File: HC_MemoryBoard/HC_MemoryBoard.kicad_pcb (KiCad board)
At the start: 2 copper layers, 100 x 100 mm, 607 parts, among them IC1 HM62256BLP, IC2 74HC30, IC3 74HC138, IC4 74HC32, IC5 74HC541, J1 Expantion_Connector, J2 Conn_01x02_Pin, J3 Conn_01x08_Pin, J4 Expantion_Connector, J5 Conn_01x08_Pin, J6 Conn_01x02_Pin, J7 Conn_01x02_Pin, SW1 SW_DIP_x08

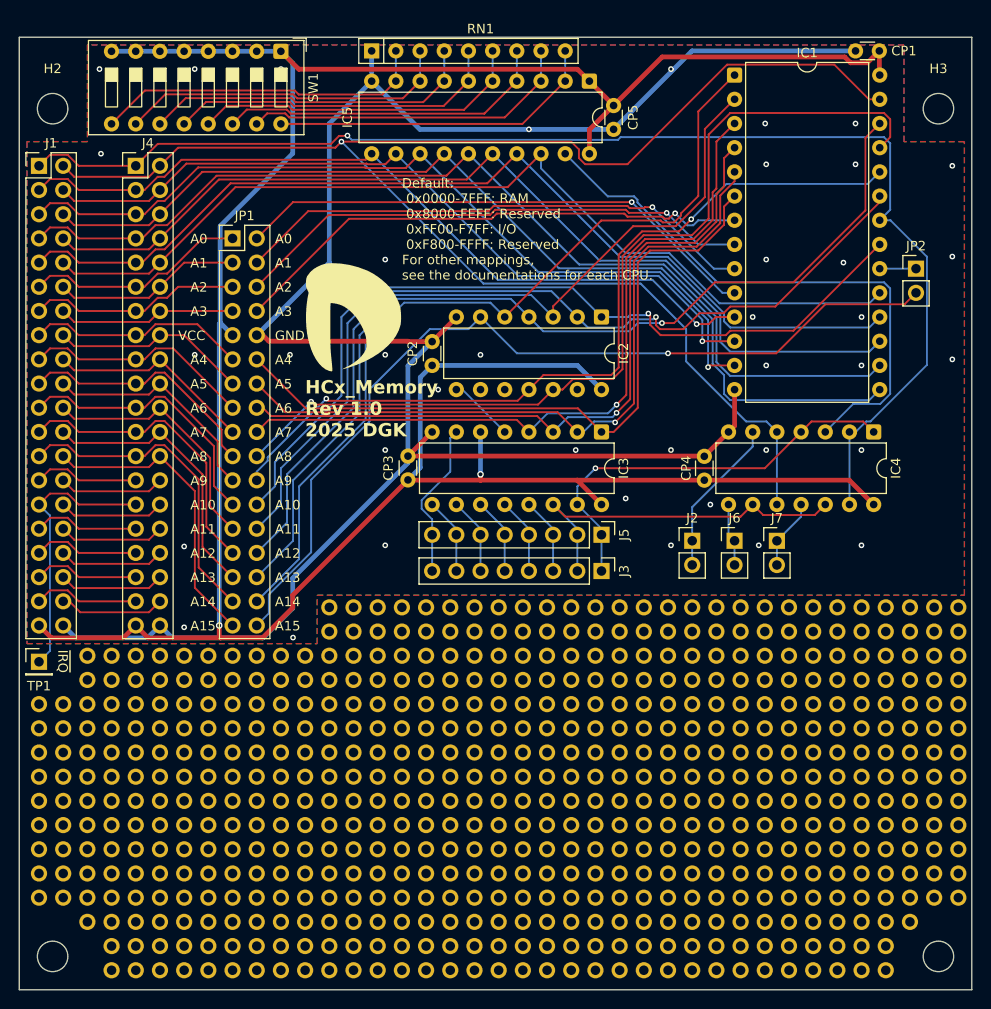
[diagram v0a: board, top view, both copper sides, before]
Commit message: Memboardv2.0
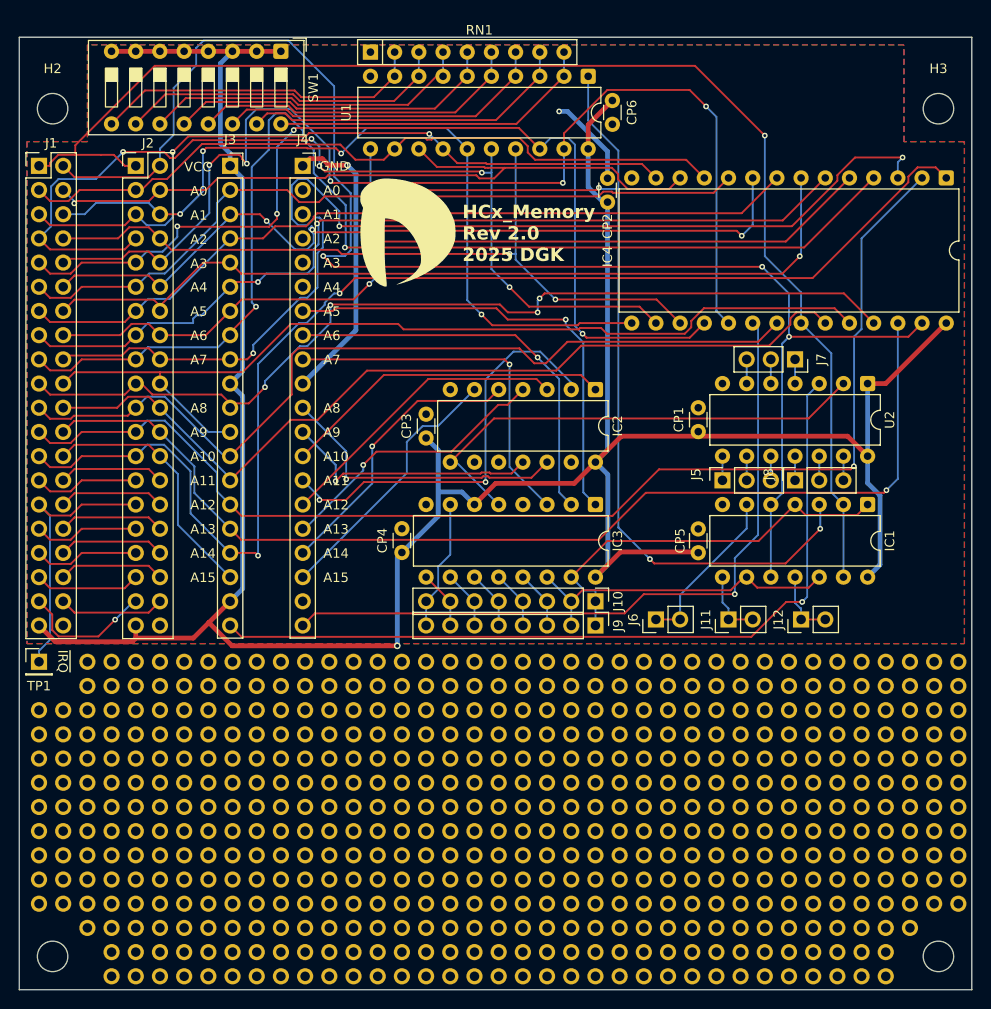
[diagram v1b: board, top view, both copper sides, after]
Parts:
- removed IC5: 74HC541, Package_DIP:DIP-20_W7.62mm
- removed JP1: Conn_02x17_Counter_Clockwise, Connector_PinHeader_2.54mm:PinHeader_2x17_P2.54mm_Vertical
- removed JP2: Jumper_2_Bridged, Connector_PinHeader_2.54mm:PinHeader_1x02_P2.54mm_Vertical
- removed REF** (x4): ThroughHole_d1.0_D1.7, ThroughHole:ThroughHole_d1.0_D1.7
- removed the REF**14 at (85.1, 114.9)
- removed the REF**14 at (82.5, 112.4)
- removed the REF**14 at (82.5, 109.9)
- removed the REF**15 at (87.6, 114.9)
- removed the REF**15 at (85.1, 112.4)
- removed the REF**15 at (85.1, 109.9)
- removed the REF**16 at (87.6, 112.4)
- removed the REF**16 at (87.6, 109.9)
- removed the REF**16 at (90.2, 114.9)
- removed the REF**17 at (92.7, 114.9)
- removed the REF**17 at (90.2, 112.4)
- removed the REF**17 at (90.2, 109.9)
- removed the REF**18 at (92.7, 112.4)
- removed the REF**18 at (95.2, 114.9)
- removed the REF**18 at (92.7, 109.9)
- removed the REF**19 at (95.2, 109.9)
- removed the REF**19 at (95.2, 112.4)
- removed the REF**19 at (97.8, 114.9)
- removed the REF**20 at (97.8, 112.4)
- removed the REF**20 at (97.8, 109.9)
- removed the REF**20 at (100.3, 114.9)
- removed the REF**21 at (100.3, 109.9)
- removed the REF**21 at (102.9, 114.9)
- removed the REF**21 at (100.3, 112.4)
- removed the REF**22 at (102.9, 112.4)
- removed the REF**22 at (102.9, 109.9)
- removed the REF**22 at (105.4, 114.9)
- removed the REF**23 at (108.0, 114.9)
- removed the REF**23 at (105.4, 112.4)
- removed the REF**23 at (105.4, 109.9)
- removed the REF**24 at (108.0, 109.9)
- removed the REF**24 at (110.5, 114.9)
- removed the REF**24 at (108.0, 112.4)
- removed the REF**25 at (110.5, 109.9)
- removed the REF**25 at (110.5, 112.4)
- removed the REF**25 at (113.0, 114.9)
- removed the REF**26 at (113.0, 112.4)
- removed the REF**26 at (113.0, 109.9)
- removed the REF**26 at (115.6, 114.9)
- removed the REF**27 at (115.6, 109.9)
- removed the REF**27 at (115.6, 112.4)
- removed the REF**27 at (118.1, 114.9)
- removed the REF**28 at (118.1, 112.4)
- removed the REF**28 at (118.1, 109.9)
- removed the REF**28 at (120.7, 114.9)
- removed the REF**29 at (123.2, 114.9)
- removed the REF**29 at (120.7, 109.9)
- removed the REF**29 at (120.7, 112.4)
- removed the REF**30 at (125.7, 114.9)
- removed the REF**30 at (123.2, 109.9)
- removed the REF**30 at (123.2, 112.4)
- removed the REF**31 at (128.3, 114.9)
- removed the REF**31 at (125.7, 109.9)
- removed the REF**31 at (125.7, 112.4)
- removed the REF**32 at (130.8, 114.9)
- removed the REF**32 at (128.3, 109.9)
- removed the REF**32 at (128.3, 112.4)
- removed the REF**33 at (130.8, 112.4)
- removed the REF**33 at (130.8, 109.9)
- removed the REF**33 at (133.3, 114.9)
- removed the REF**34 at (133.3, 109.9)
- removed the REF**34 at (135.9, 114.9)
- removed the REF**34 at (133.3, 112.4)
- removed the REF**35 at (138.4, 114.9)
- removed the REF**35 at (135.9, 109.9)
- removed the REF**35 at (135.9, 112.4)
- removed the REF**36 at (138.4, 109.9)
- removed the REF**36 at (138.4, 112.4)
- removed the REF**36 at (141.0, 114.9)
- removed the REF**37 at (141.0, 109.9)
- removed the REF**37 at (141.0, 112.4)
- removed the REF**37 at (143.5, 114.9)
- removed the REF**38 at (143.5, 112.4)
- removed the REF**38 at (146.1, 114.9)
- removed the REF**38 at (143.5, 109.9)
- removed the REF**39 at (146.1, 112.4)
- removed the REF**39 at (148.6, 114.9)
- removed the REF**39 at (146.1, 109.9)
- added CP1: 0.1u, Capacitor_THT:C_Disc_D3.0mm_W1.6mm_P2.50mm, F.Cu at (121.3, 91.4)
- added J3: Changer, Connector_PinSocket_2.54mm:PinSocket_1x20_P2.54mm_Vertical, F.Cu at (72.1, 63.5)
- added J4: Changer, Connector_PinSocket_2.54mm:PinSocket_1x20_P2.54mm_Vertical, F.Cu at (79.8, 63.5)
- added J5: Conn_01x03_Pin, Connector_PinSocket_2.54mm:PinSocket_1x03_P2.54mm_Vertical, F.Cu at (123.8, 96.5)
- added J7: Conn_01x03_Pin, Connector_PinSocket_2.54mm:PinSocket_1x03_P2.54mm_Vertical, F.Cu at (131.4, 83.8)
- added J8: Conn_01x03_Pin, Connector_PinSocket_2.54mm:PinSocket_1x03_P2.54mm_Vertical, F.Cu at (131.4, 96.5)
- added REF**14: ThroughHole_d1.0_D1.7, ThroughHole:ThroughHole_d1.0_D1.7, F.Cu at (85.1, 115.6)
- added REF**15: ThroughHole_d1.0_D1.7, ThroughHole:ThroughHole_d1.0_D1.7, F.Cu at (87.6, 115.6)
- added REF**16: ThroughHole_d1.0_D1.7, ThroughHole:ThroughHole_d1.0_D1.7, F.Cu at (90.2, 115.6)
- added REF**17: ThroughHole_d1.0_D1.7, ThroughHole:ThroughHole_d1.0_D1.7, F.Cu at (92.7, 115.6)
- added REF**18: ThroughHole_d1.0_D1.7, ThroughHole:ThroughHole_d1.0_D1.7, F.Cu at (95.2, 115.6)
- added REF**19: ThroughHole_d1.0_D1.7, ThroughHole:ThroughHole_d1.0_D1.7, F.Cu at (97.8, 115.6)
- added REF**20: ThroughHole_d1.0_D1.7, ThroughHole:ThroughHole_d1.0_D1.7, F.Cu at (100.3, 115.6)
- added REF**21: ThroughHole_d1.0_D1.7, ThroughHole:ThroughHole_d1.0_D1.7, F.Cu at (102.9, 115.6)
- added REF**22: ThroughHole_d1.0_D1.7, ThroughHole:ThroughHole_d1.0_D1.7, F.Cu at (105.4, 115.6)
- added REF**23: ThroughHole_d1.0_D1.7, ThroughHole:ThroughHole_d1.0_D1.7, F.Cu at (108.0, 115.6)
- added REF**24: ThroughHole_d1.0_D1.7, ThroughHole:ThroughHole_d1.0_D1.7, F.Cu at (110.5, 115.6)
- added REF**25: ThroughHole_d1.0_D1.7, ThroughHole:ThroughHole_d1.0_D1.7, F.Cu at (113.0, 115.6)
- added REF**26: ThroughHole_d1.0_D1.7, ThroughHole:ThroughHole_d1.0_D1.7, F.Cu at (115.6, 115.6)
- added REF**27: ThroughHole_d1.0_D1.7, ThroughHole:ThroughHole_d1.0_D1.7, F.Cu at (118.1, 115.6)
- added REF**28: ThroughHole_d1.0_D1.7, ThroughHole:ThroughHole_d1.0_D1.7, F.Cu at (120.7, 115.6)
- added REF**29: ThroughHole_d1.0_D1.7, ThroughHole:ThroughHole_d1.0_D1.7, F.Cu at (123.2, 115.6)
- added REF**30: ThroughHole_d1.0_D1.7, ThroughHole:ThroughHole_d1.0_D1.7, F.Cu at (125.7, 115.6)
- added REF**31: ThroughHole_d1.0_D1.7, ThroughHole:ThroughHole_d1.0_D1.7, F.Cu at (128.3, 115.6)
- added REF**32: ThroughHole_d1.0_D1.7, ThroughHole:ThroughHole_d1.0_D1.7, F.Cu at (130.8, 115.6)
- added REF**33: ThroughHole_d1.0_D1.7, ThroughHole:ThroughHole_d1.0_D1.7, F.Cu at (133.3, 115.6)
- added REF**34: ThroughHole_d1.0_D1.7, ThroughHole:ThroughHole_d1.0_D1.7, F.Cu at (135.9, 115.6)
- added REF**35: ThroughHole_d1.0_D1.7, ThroughHole:ThroughHole_d1.0_D1.7, F.Cu at (138.4, 115.6)
- added REF**36: ThroughHole_d1.0_D1.7, ThroughHole:ThroughHole_d1.0_D1.7, F.Cu at (141.0, 115.6)
- added REF**37: ThroughHole_d1.0_D1.7, ThroughHole:ThroughHole_d1.0_D1.7, F.Cu at (143.5, 115.6)
- added REF**38: ThroughHole_d1.0_D1.7, ThroughHole:ThroughHole_d1.0_D1.7, F.Cu at (146.1, 115.6)
- added REF**39: ThroughHole_d1.0_D1.7, ThroughHole:ThroughHole_d1.0_D1.7, F.Cu at (148.6, 115.6)
- added REF**432: ThroughHole_d1.0_D1.7, ThroughHole:ThroughHole_d1.0_D1.7, F.Cu at (57.1, 143.5)
- added REF**466: ThroughHole_d1.0_D1.7, ThroughHole:ThroughHole_d1.0_D1.7, F.Cu at (143.5, 143.5)
- added U1: 74HC573, Package_DIP:DIP-20_W7.62mm, F.Cu at (109.7, 54.1)
- added U2: 74HC00, Package_DIP:DIP-14_W7.62mm, F.Cu at (139.1, 86.4)
- moved CP2 32.7 mm to (111.8, 67.3), turned to 90 degrees
- moved IC4 24.7 mm to (147.3, 64.8), turned to -90 degrees
- moved G*** 10.6 mm to (90.8, 70.5)
- moved J6 9.10 mm to (116.8, 111.1), turned to 90 degrees
- moved J12 8.64 mm to (132.1, 111.1), turned to 90 degrees
- moved J11 8.28 mm to (124.5, 111.1), turned to 90 degrees
- moved CP3 7.65 mm to (92.7, 92.1)
- moved CP4 7.65 mm to (90.2, 104.1)
- moved CP5 7.65 mm to (121.3, 104.1)
- moved IC3 7.65 mm to (110.5, 99.1)
- moved IC1 7.65 mm to (139.1, 99.1)
- moved IC2 7.65 mm to (110.5, 87.0)
- moved J10 7.01 mm to (110.5, 109.2)
- moved J9 5.76 mm to (110.5, 111.8)
- moved REF**352 0.64 mm to (52.1, 138.4)
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- renumbered CP1 to CP2, CP2 to CP3, CP3 to CP4, CP4 to CP5, CP5 to CP6, IC4 to IC1, IC1 to IC4, J5 to J10, J6 to J11, J7 to J12, J4 to J2, J2 to J6, J3 to J9
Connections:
- net Net-(IC3-~{E1}) renamed /7430
- IC3 pad 1: /A4 -> /A5
- IC3 pad 2: /A5 -> /A6
- IC3 pad 3: /A6 -> /A7
- IC3 pad 4: /A7 -> GND
- IC4 pad 1: /A14 -> /AD14
- IC4 pad 10: /A0 -> /AD0
- IC4 pad 2: /A12 -> /AD12
- IC4 pad 20: Net-(IC1-~{CS}) -> /~{RAM_CE}
- IC4 pad 21: /A10 -> /AD10
- IC4 pad 23: /A11 -> /AD11
- IC4 pad 24: /A9 -> /AD9
- IC4 pad 25: /A8 -> /AD8
- IC4 pad 26: /A13 -> /AD13
- IC4 pad 3: /A7 -> /AD7
- IC4 pad 4: /A6 -> /AD6
- IC4 pad 5: /A5 -> /AD5
- IC4 pad 6: /A4 -> /AD4
- IC4 pad 7: /A3 -> /AD3
- IC4 pad 8: /A2 -> /AD2
- IC4 pad 9: /A1 -> /AD1
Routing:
- net GND: track 217.6 -> 40.5 mm, vias 39 -> 2
- net /AD14: track 34.0 -> 133.7 mm, vias 0 -> 2
- net /AD6: track 24.3 -> 124.0 mm, vias 0 -> 2
- net /AD7: track 21.9 -> 119.1 mm, vias 0 -> 3
- net /AD12: track 31.4 -> 127.7 mm, vias 0 -> 1
- net Net-(J3-Pin_20): track 0.00 -> 85.7 mm, vias 0 -> 1
- net /AD13: track 29.5 -> 113.9 mm, vias 0 -> 1
- net /~{RAM_CE}: track 0.00 -> 76.4 mm, vias 0 -> 1
- net /AD9: track 24.4 -> 98.5 mm
- net /A4: track 73.6 -> 0.00 mm
- net /AD5: track 20.8 -> 93.4 mm, vias 0 -> 2
- net /AD8: track 26.3 -> 98.9 mm, vias 0 -> 4
- net /A13: track 101.0 -> 29.5 mm
- net /AD3: track 18.7 -> 90.0 mm, vias 0 -> 1
- net /AD4: track 23.3 -> 93.2 mm, vias 0 -> 2
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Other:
- board text added: "HCx_Memory Rev 2.0 2025 DGK"
- board text removed: "Default: 0x0000-7FFF: RAM 0x8000-FEFF: Reserved 0xFF00-F7FF: I/O 0xF800-FFFF: Reserved For other mappings, see the documentations for each CPU."
- board text removed: "HCx_Memory Rev 1.0 2025 DGK"
